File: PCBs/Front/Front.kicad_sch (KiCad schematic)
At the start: 2 parts, among them J1 PWR, J2 CAP_TOUCH

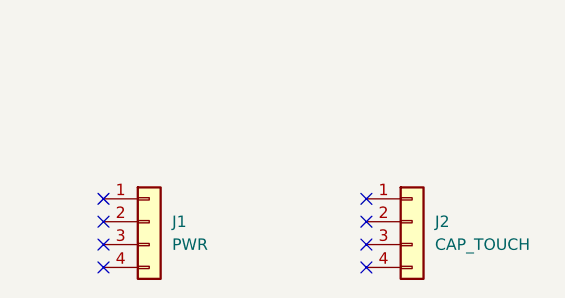
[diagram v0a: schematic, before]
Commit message: Cleaned up schematic and generated pdfs
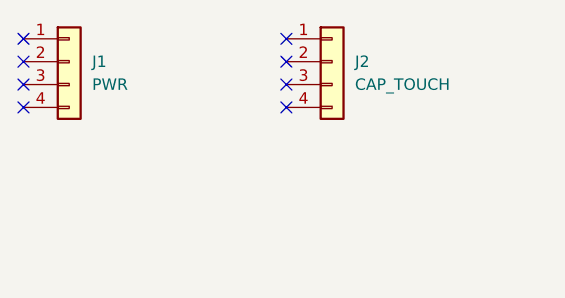
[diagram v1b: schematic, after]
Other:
- moved on the sheet: J1, J2
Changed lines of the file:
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@@
 (kicad_sch (version 20230121) (generator eeschema)
-  (paper "A4")
-  (no_connect (at 119.38 80.01))
-  (no_connect (at 119.38 85.09))
-  (no_connect (at 119.38 82.55))
-  (no_connect (at 119.38 77.47))
-  (no_connect (at 90.17 80.01))
-  (no_connect (at 90.17 85.09))
-  (no_connect (at 90.17 82.55))
-  (no_connect (at 90.17 77.47))
-  (symbol (lib_id "Connector_Generic:Conn_01x04") (at 124.46 80.01 0) (unit 1)
+  (paper "A5")
+  (no_connect (at 110.49 62.23))
+  (no_connect (at 110.49 67.31))
+  (no_connect (at 110.49 64.77))
+  (no_connect (at 110.49 59.69))
+  (no_connect (at 81.28 62.23))
+  (no_connect (at 81.28 67.31))
+  (no_connect (at 81.28 64.77))
+  (no_connect (at 81.28 59.69))
+  (symbol (lib_id "Connector_Generic:Conn_01x04") (at 115.57 62.23 0) (unit 1)
     (in_bom yes) (on_board yes) (dnp no) (fields_autoplaced)
-    (property "Reference" "J2" (at 127 80.01 0)
+    (property "Reference" "J2" (at 118.11 62.23 0)
       (effects (font (size 1.27 1.27)) (justify left))
     )
-    (property "Value" "CAP_TOUCH" (at 127 82.55 0)
+    (property "Value" "CAP_TOUCH" (at 118.11 64.77 0)
       (effects (font (size 1.27 1.27)) (justify left))
     )
-    (property "Footprint" "fp:PinHeader_1x04_P2.54mm_Vertical_SMD_Both" (at 124.46 80.01 0)
+    (property "Footprint" "fp:PinHeader_1x04_P2.54mm_Vertical_SMD_Both" (at 115.57 62.23 0)
       (effects (font (size 1.27 1.27)) hide)
     )
-    (property "Datasheet" "~" (at 124.46 80.01 0)
+    (property "Datasheet" "~" (at 115.57 62.23 0)
       (effects (font (size 1.27 1.27)) hide)
     )
@@
     )
   )
-  (symbol (lib_id "Connector_Generic:Conn_01x04") (at 95.25 80.01 0) (unit 1)
+  (symbol (lib_id "Connector_Generic:Conn_01x04") (at 86.36 62.23 0) (unit 1)
     (in_bom yes) (on_board yes) (dnp no) (fields_autoplaced)
-    (property "Reference" "J1" (at 97.79 80.01 0)
+    (property "Reference" "J1" (at 88.9 62.23 0)
       (effects (font (size 1.27 1.27)) (justify left))
     )
-    (property "Value" "PWR" (at 97.79 82.55 0)
+    (property "Value" "PWR" (at 88.9 64.77 0)
       (effects (font (size 1.27 1.27)) (justify left))
     )
-    (property "Footprint" "fp:PinHeader_1x04_P2.54mm_Vertical_SMD_Both" (at 95.25 80.01 0)
+    (property "Footprint" "fp:PinHeader_1x04_P2.54mm_Vertical_SMD_Both" (at 86.36 62.23 0)
       (effects (font (size 1.27 1.27)) hide)
     )
-    (property "Datasheet" "~" (at 95.25 80.01 0)
+    (property "Datasheet" "~" (at 86.36 62.23 0)
       (effects (font (size 1.27 1.27)) hide)
     )
